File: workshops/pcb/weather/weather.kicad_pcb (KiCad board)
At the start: 2 copper layers, 5 parts, among them J2 Conn_01x04_Female, J3 Conn_01x03_Female, J4 Conn_01x03_Female

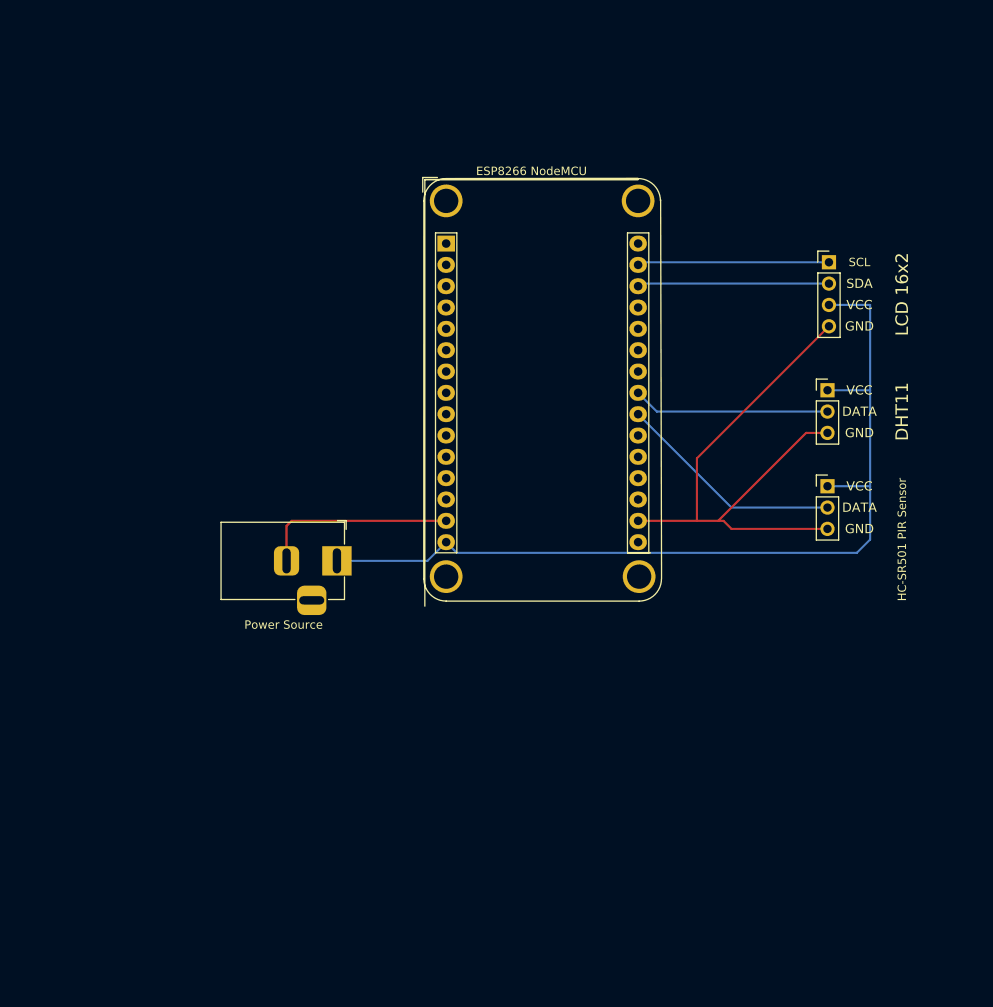
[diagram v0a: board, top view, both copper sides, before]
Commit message: Update custom_logo.kicad_mod, fp-info-cache, and 7 more files...
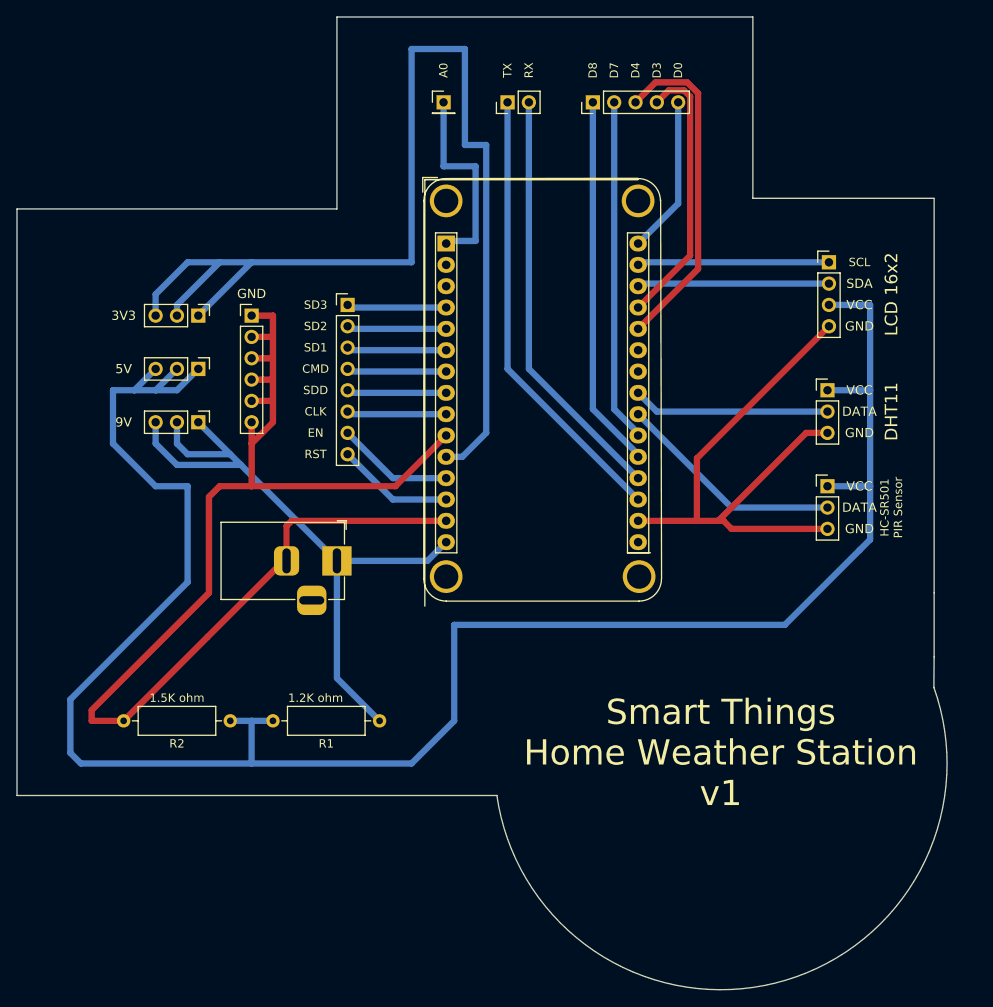
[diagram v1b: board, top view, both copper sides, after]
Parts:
- added J10: Conn_01x03_Female, Connector_PinHeader_2.54mm:PinHeader_1x03_P2.54mm_Vertical, F.Cu at (97.8, 108.0)
- added J11: Conn_01x03_Female, Connector_PinHeader_2.54mm:PinHeader_1x03_P2.54mm_Vertical, F.Cu at (97.8, 101.6)
- added J12: Conn_01x06_Female, Connector_PinHeader_2.54mm:PinHeader_1x06_P2.54mm_Vertical, F.Cu at (104.1, 101.6)
- added J5: Conn_01x08_Female, Connector_PinHeader_2.54mm:PinHeader_1x08_P2.54mm_Vertical, F.Cu at (115.6, 100.3)
- added J6: Conn_01x01_Female, Connector_PinHeader_2.54mm:PinHeader_1x01_P2.54mm_Vertical, F.Cu at (127.0, 76.2)
- added J7: Conn_01x02_Female, Connector_PinHeader_2.54mm:PinHeader_1x02_P2.54mm_Vertical, F.Cu at (134.6, 76.2)
- added J8: Conn_01x05_Female, Connector_PinHeader_2.54mm:PinHeader_1x05_P2.54mm_Vertical, F.Cu at (144.8, 76.2)
- added J9: Conn_01x03_Female, Connector_PinHeader_2.54mm:PinHeader_1x03_P2.54mm_Vertical, F.Cu at (97.8, 114.3)
- added R1: 1.2K ohm, Resistor_THT:R_Axial_DIN0309_L9.0mm_D3.2mm_P12.70mm_Horizontal, F.Cu at (119.4, 149.9)
- added R2: 1.5K ohm, Resistor_THT:R_Axial_DIN0309_L9.0mm_D3.2mm_P12.70mm_Horizontal, F.Cu at (101.6, 149.9)
- J1: renamed from Power Source
- U1: renamed from ESP8266 NodeMCU
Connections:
- J1 pad 2: Net-(J1-Pad2) -> GND
- J2 pad 3: +9V -> +5V
- J3 pad 1: +9V -> +5V
- J4 pad 1: +9V -> +5V
- U1 pad 10: Net-(U1-Pad10) -> GND
- U1 pad 11: Net-(U1-Pad11) -> +3V3
- U1 pad 14: Net-(J1-Pad2) -> GND
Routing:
- net +5V: track 0.00 -> 240.4 mm
- net GND: track 70.0 -> 224.8 mm
- net +3V3: track 0.00 -> 138.0 mm
- net Net-(J7-Pad1): track 0.00 -> 53.7 mm
- net Net-(J7-Pad2): track 0.00 -> 50.1 mm
- net Net-(J8-Pad1): track 0.00 -> 44.5 mm
- net Net-(J8-Pad2): track 0.00 -> 40.9 mm
- net Net-(J8-Pad3): track 0.00 -> 40.0 mm
- net Net-(J8-Pad4): track 0.00 -> 32.6 mm
- net +9V: track 108.6 -> 81.6 mm
- net Net-(J6-Pad1): track 0.00 -> 23.9 mm
- net Net-(J1-Pad2): track 23.4 -> 0.00 mm
- net Net-(J8-Pad5): track 0.00 -> 18.8 mm
- net Net-(J5-Pad7): track 0.00 -> 14.0 mm
- net Net-(J5-Pad8): track 0.00 -> 14.0 mm
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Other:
- board outline added: 110.8 x 115.8 mm
- board text added: "3V3"
- board text added: "5V"
- board text added: "9V"
- board text added: "A0"
- board text added: "CLK"
- board text added: "CMD"
- board text added: "D0"
- board text added: "D3"
- board text added: "D4"
- board text added: "D7"
- board text added: "D8"
- board text added: "EN"
- board text added: "RST"
- board text added: "RX"
- board text added: "SD1"
- board text added: "SD2"
- board text added: "SD3"
- board text added: "SDD"
- board text added: "Smart Things Home Weather Station v1"
- board text added: "TX"
